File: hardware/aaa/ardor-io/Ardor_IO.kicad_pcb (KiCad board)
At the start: 2 copper layers, 100 x 80 mm, 99 parts, among them J101 PI 40-PIN HEADER, J102 CODEC AUX L / GND / R, J202 TO MIDI PANEL / 4,5, J302 TO EXP PANEL / T,R,S, J502 TO YOUR AMP CIRCUIT, J503 TO LINE PANEL / T,S, J602 TO HP PANEL / T,R,S, K501 G5V-1 DC5, Q501 2N7002, U201 H11L1M, U301 ADS1115IDGS, U401 OPA2320AIDR, U402 OPA2320AIDR, U501 OPA2320AIDR, U601 TPA6132A2RTER

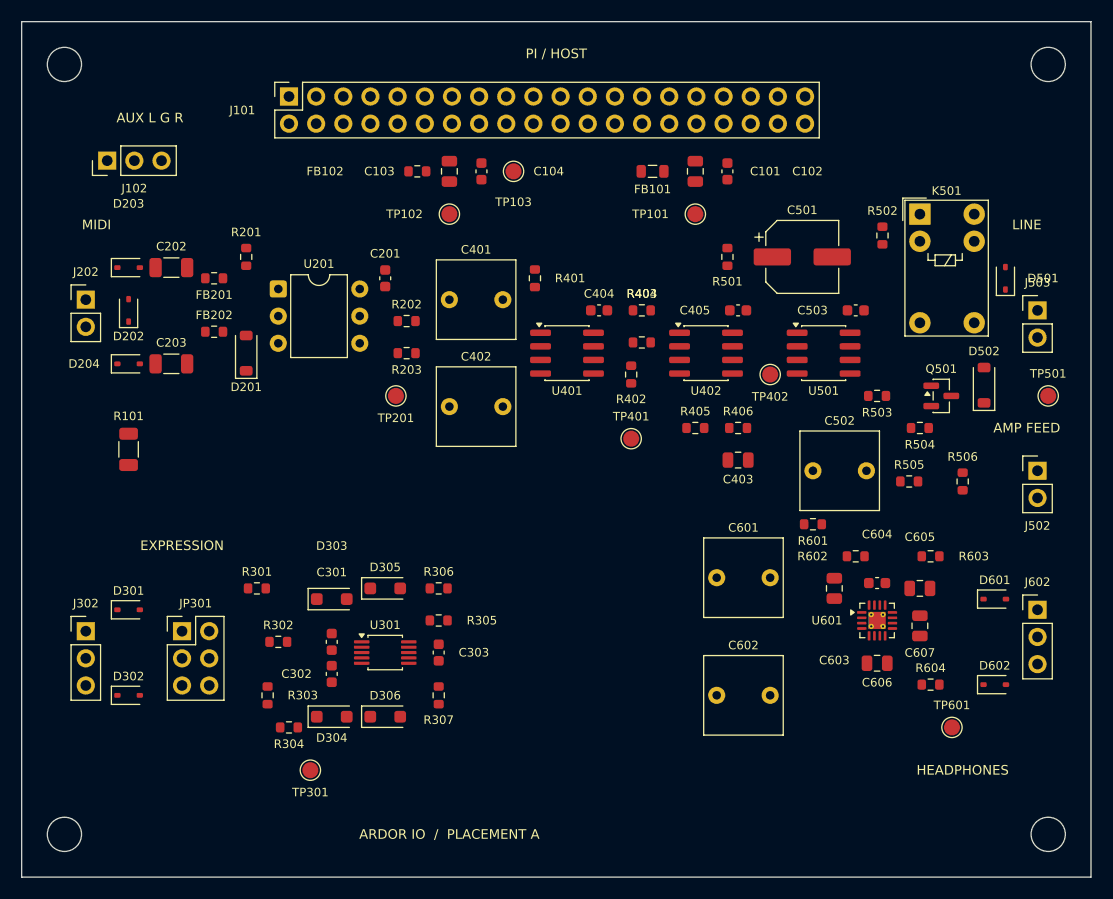
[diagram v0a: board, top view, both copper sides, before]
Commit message: feat: kicad PCB
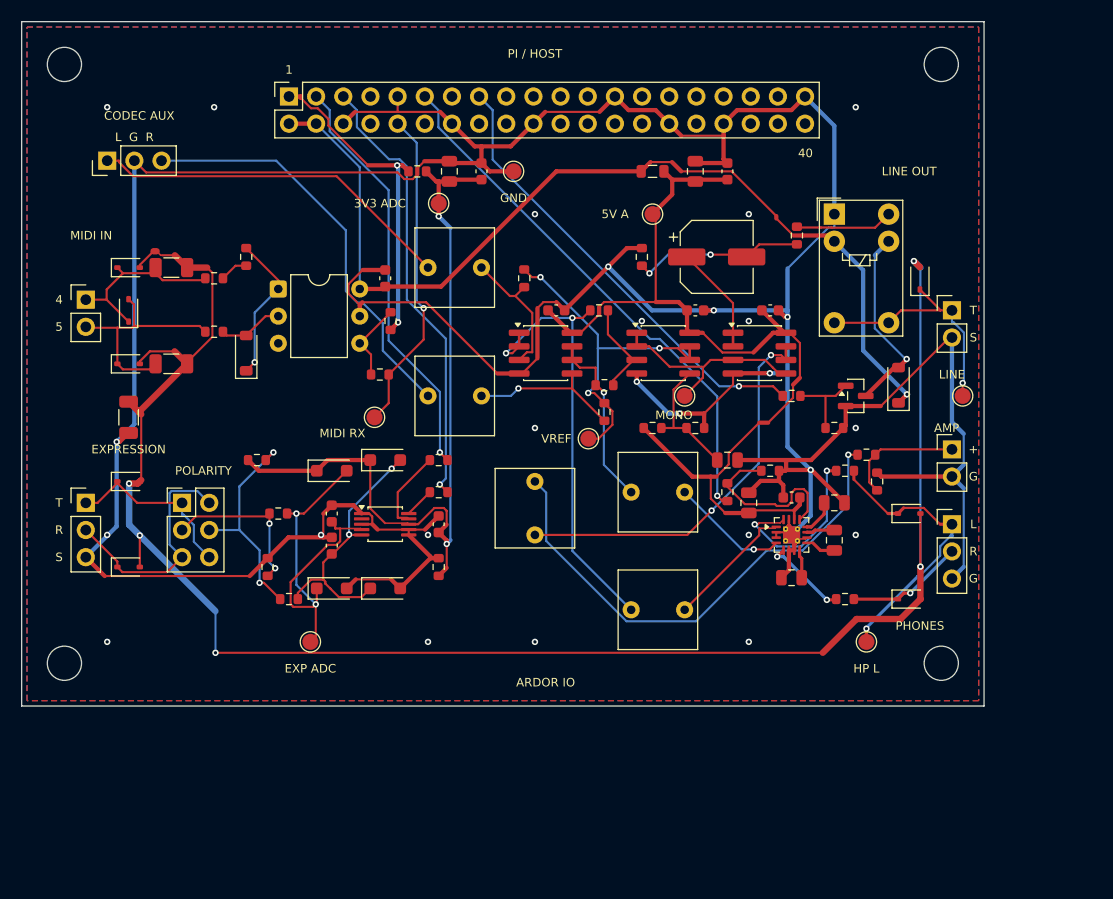
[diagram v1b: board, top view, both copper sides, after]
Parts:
- H1, H2, H3, H4: footprint MountingHole_3.2mm_M3 -> MountingHole:MountingHole_3.2mm_M3
- moved C502 26.7 mm to (98.0, 98.0), turned to 90 degrees
- moved H4 18.9 mm to (136.0, 110.0)
- moved H3 16.0 mm to (54.0, 110.0)
- moved C301 12.0 mm to (79.0, 96.0)
- moved C302 12.0 mm to (79.0, 99.0)
- moved C303 12.0 mm to (89.0, 97.0)
- moved D301 12.0 mm to (60.0, 93.0)
- moved D302 12.0 mm to (60.0, 101.0)
- moved D303 12.0 mm to (79.0, 92.0)
- moved D304 12.0 mm to (79.0, 103.0)
- moved D305 12.0 mm to (84.0, 91.0)
- moved D306 12.0 mm to (84.0, 103.0)
- moved J302 12.0 mm to (56.0, 95.0)
- moved JP301 12.0 mm to (65.0, 95.0)
- moved R301 12.0 mm to (72.0, 91.0)
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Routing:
- net GND: track 0.00 -> 407.0 mm, vias 0 -> 26
- net CHASSIS: track 0.00 -> 166.6 mm, vias 0 -> 5
- net +5V_PI: track 0.00 -> 90.4 mm, vias 0 -> 1
- net +5V_A: track 0.00 -> 90.0 mm
- net +3V3_ADC: track 0.00 -> 72.4 mm, vias 0 -> 2
- net HP_ENABLE: track 0.00 -> 50.3 mm, vias 0 -> 1
- net /05 / Line and amp feed/AMP_AC: track 0.00 -> 47.4 mm, vias 0 -> 1
- net LINE_ENABLE: track 0.00 -> 42.7 mm, vias 0 -> 1
- net PI_SCL: track 0.00 -> 42.1 mm, vias 0 -> 1
- net BUF_L: track 0.00 -> 41.9 mm, vias 0 -> 2
- net PI_SDA: track 0.00 -> 39.1 mm, vias 0 -> 1
- net AUX_R: track 0.00 -> 38.9 mm
- net /05 / Line and amp feed/AMP_BUF: track 0.00 -> 37.2 mm, vias 0 -> 2
- net EXP_ADC: track 0.00 -> 37.0 mm, vias 0 -> 2
- net AUX_L: track 0.00 -> 34.2 mm
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- added copper zone on B.Cu, net GND
- added copper zone on F.Cu, net GND
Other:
- board size 100 x 80 mm -> 90 x 64 mm
- board text added: "+"
- board text added: "1"
- board text added: "3V3 ADC"
- board text added: "4"
- board text added: "40"
- board text added: "5"
- board text added: "5V A"
- board text added: "AMP"
- board text added: "ARDOR IO"
- board text added: "CODEC AUX"
- board text added: "EXP ADC"
- board text added: "G"
- board text added: "GND"
- board text added: "HP L"
- board text added: "JP301: NORMAL 1-3 / 2-4; REVERSE 3-5 / 4-6"
- board text added: "L"
- board text added: "L G R"
- board text added: "LINE OUT"
- board text added: "MIDI IN"
- board text added: "MIDI RX"
- board text added: "MONO"
- board text added: "PHONES"
- board text added: "POLARITY"
- board text added: "R"
- board text added: "S"
- board text added: "T"
- board text added: "VREF"
- board text removed: "100 x 80 mm / UNROUTED"
- board text removed: "AMP FEED"
- board text removed: "ARDOR IO / PLACEMENT A"
- board text removed: "AUDIO BUFFERS"
- board text removed: "AUX L G R"
- board text removed: "CONTROL ADC"
- board text removed: "HEADPHONES"
- board text removed: "MIDI"
- board text removed: "MIDI ISOLATION CORRIDOR"
- board text removed: "RELAY"
